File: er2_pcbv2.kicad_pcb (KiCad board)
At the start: 2 copper layers, 83.8 x 57.5 mm, 52 parts, among them IC1 LM2596S, IC2 XC6206, IC3 L293DD, IC4 L293DD, IC5 MMA7455, P1 CONN_3X2, P10 CONN_5, P2 CONN_3X2, P3 CONN_13X2, P4 CONN_2, P5 CONN_2, P6 CONN_2, P7 CONN_2, P8 CONN_2, P9 CONN_2, U1 74HC595

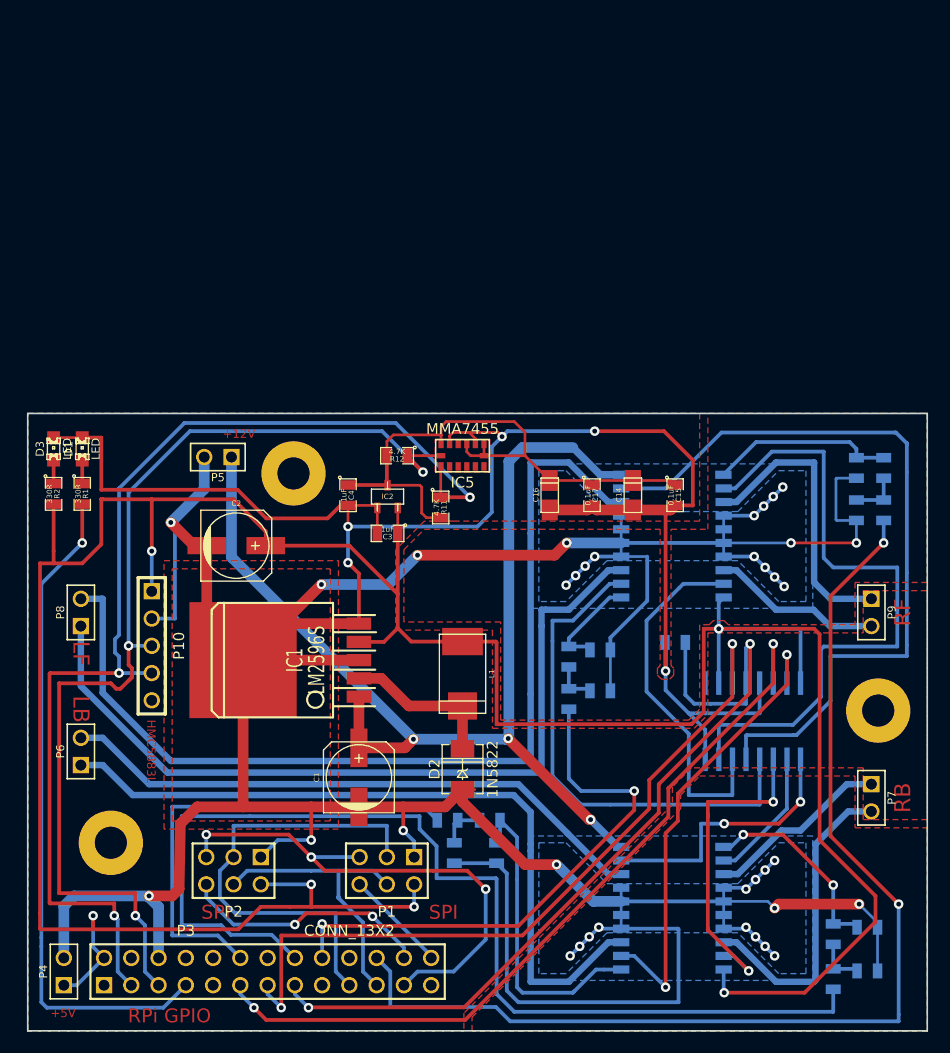
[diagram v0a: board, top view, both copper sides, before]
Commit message: preliminary PCB components placement
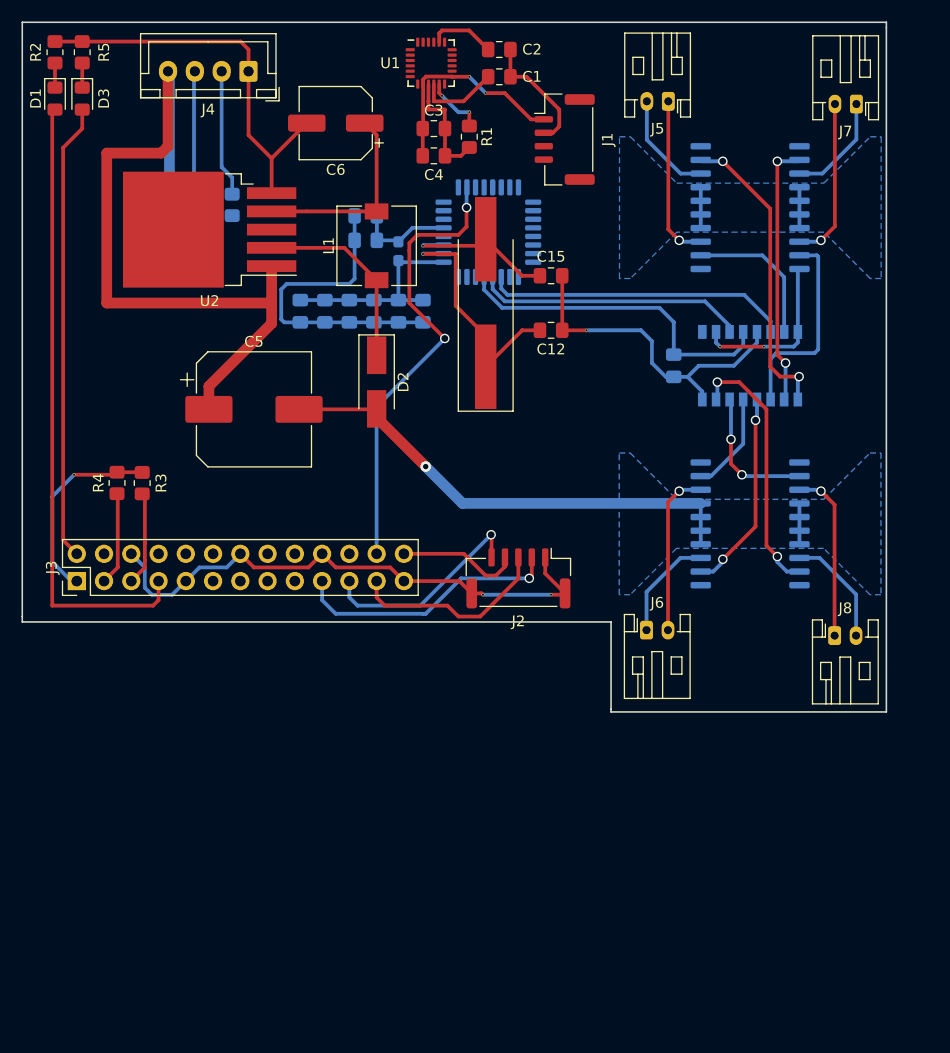
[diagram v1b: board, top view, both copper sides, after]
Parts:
- removed ? (x3): , mnt_hole
- removed IC1: LM2596S, TO263-5
- removed IC2: XC6206, sot23
- removed IC3, IC4: L293DD, -SO20-2
- removed IC5: MMA7455, LGA_14
- removed P1, P2: CONN_3X2, pin_array_3x2
- removed P10: CONN_5, PIN_ARRAY_5x1
- removed P3: CONN_13X2, pin_array_13x2
- removed P4, P5, P6, P7, P8, P9: CONN_2, PIN_ARRAY_2X1
- removed R11, R12: 4.7K, SM0805
- added J1: HMC5883L, Connector_JST:JST_GH_BM04B-GHS-TBT_1x04-1MP_P1.25mm_Vertical, F.Cu at (158.0, 50.8)
- added J2: SPI1, Connector_JST:JST_GH_BM05B-GHS-TBT_1x05-1MP_P1.25mm_Vertical, F.Cu at (153.7, 91.7)
- added J3: raspberry_b_plus_header, Connector_PinHeader_2.54mm:PinHeader_2x13_P2.54mm_Vertical, F.Cu at (112.5, 91.9)
- added J4: Power, Connector_JST:JST_XH_B4B-XH-A_1x04_P2.50mm_Vertical, F.Cu at (128.5, 44.5)
- added J5: WHL_LF, Connector_JST:JST_PH_S2B-PH-K_1x02_P2.00mm_Horizontal, F.Cu at (167.6, 47.2)
- added J6: WHL_LB, Connector_JST:JST_PH_S2B-PH-K_1x02_P2.00mm_Horizontal, F.Cu at (165.6, 96.5)
- added J7: WHL_RF, Connector_JST:JST_PH_S2B-PH-K_1x02_P2.00mm_Horizontal, F.Cu at (185.2, 47.5)
- added J8: WHL_RB, Connector_JST:JST_PH_S2B-PH-K_1x02_P2.00mm_Horizontal, F.Cu at (183.1, 97.0)
- added L2: 39nH, Inductor_SMD:L_0603_1608Metric_Pad1.05x0.95mm_HandSolder, B.Cu at (142.5, 61.2)
- added U2: LM2596S-5, Package_TO_SOT_SMD:TO-263-5_TabPin3, F.Cu at (124.9, 59.2)
- added U3: STM32F030K6Tx, Package_QFP:LQFP-32_7x7mm_P0.8mm, B.Cu at (150.9, 59.4)
- added U4: 74HC595, Package_SO:SOP-16_4.4x10.4mm_P1.27mm, B.Cu at (175.3, 71.9)
- added U5: L293DD, Package_SO:SOP-20_7.5x12.8mm_P1.27mm, B.Cu at (175.3, 57.1)
- added U6: L293DD, Package_SO:SOP-20_7.5x12.8mm_P1.27mm, B.Cu at (175.3, 86.6)
- added Y1: 8Mhz, Crystal:Crystal_SMD_HC49-SD_HandSoldering, F.Cu at (150.6, 66.0)
- C1: value 100uF -> 0.1uF; footprint c_elec_6.3x7.7 -> Capacitor_SMD:C_0805_2012Metric_Pad1.18x1.45mm_HandSolder
- C10, C8, C9: value 1uF -> 100nF; footprint SM0805 -> Capacitor_SMD:C_0805_2012Metric_Pad1.18x1.45mm_HandSolder
- C11: footprint SM0805 -> Capacitor_SMD:C_0805_2012Metric_Pad1.18x1.45mm_HandSolder
- C12: value 1uF -> 20p; footprint SM0805 -> Capacitor_SMD:C_0805_2012Metric_Pad1.18x1.45mm_HandSolder; moved to F.Cu
- C13: value 0.1uF -> 100nF; footprint SM0805 -> Capacitor_SMD:C_0805_2012Metric_Pad1.18x1.45mm_HandSolder
- C14: value 10uF -> 10nF; footprint c_tant_A -> Capacitor_SMD:C_0805_2012Metric_Pad1.18x1.45mm_HandSolder; moved to B.Cu
- C15: value 0.1uF -> 20p; footprint SM0805 -> Capacitor_SMD:C_0805_2012Metric_Pad1.18x1.45mm_HandSolder
- C16: value 10uF -> 100nF; footprint c_tant_A -> Capacitor_SMD:C_0805_2012Metric_Pad1.18x1.45mm_HandSolder; moved to B.Cu
- C17: value 0.1uF -> 1uF; footprint SM0805 -> Capacitor_SMD:C_0805_2012Metric_Pad1.18x1.45mm_HandSolder; moved to B.Cu
- C2: value 220uF -> 2.2nF; footprint c_elec_6.3x7.7 -> Capacitor_SMD:C_0805_2012Metric_Pad1.18x1.45mm_HandSolder
- C3: value 1uF -> 10nF; footprint SM0805 -> Capacitor_SMD:C_0805_2012Metric_Pad1.18x1.45mm_HandSolder
- C4: value 1uF -> 0.1uF; footprint SM0805 -> Capacitor_SMD:C_0805_2012Metric_Pad1.18x1.45mm_HandSolder
- C5: value 1uF -> 680uF; footprint SM0805 -> Capacitor_SMD:CP_Elec_10x10.5; moved to F.Cu
- C6: value 1uF -> 220uF; footprint SM0805 -> Capacitor_SMD:CP_Elec_6.3x7.7; moved to F.Cu
- C7: value 1uF -> 4.7uF; footprint SM0805 -> Capacitor_SMD:C_0805_2012Metric_Pad1.18x1.45mm_HandSolder
- D1, D3: footprint LED-0805 -> LED_SMD:LED_0805_2012Metric_Pad1.15x1.40mm_HandSolder
- D2: footprint DO-214AC(SMA) -> Diode_SMD:D_SMA_Handsoldering
- L1: footprint c_tant_X -> Inductor_SMD:L_7.3x7.3_H3.5
- R1, R2: value 330R -> 1k; footprint SM0805 -> Resistor_SMD:R_0805_2012Metric_Pad1.20x1.40mm_HandSolder
- R10, R7, R8: value 4.7K -> 10k; footprint SM0805 -> Resistor_SMD:R_0805_2012Metric_Pad1.20x1.40mm_HandSolder
- R3, R4: value 4.7K -> 4.7k; footprint SM0805 -> Resistor_SMD:R_0805_2012Metric_Pad1.20x1.40mm_HandSolder; moved to F.Cu
- R5: value 4.7K -> 1k; footprint SM0805 -> Resistor_SMD:R_0805_2012Metric_Pad1.20x1.40mm_HandSolder; moved to F.Cu
- R6, R9: value 4.7K -> 22k; footprint SM0805 -> Resistor_SMD:R_0805_2012Metric_Pad1.20x1.40mm_HandSolder
- U1: value 74HC595 -> MPU-6050; footprint -SOP-16 -> Sensor_Motion:InvenSense_QFN-24_4x4mm_P0.5mm; moved to F.Cu
- moved C6 93.2 mm to (136.7, 49.3), turned to 180 degrees
- moved R8 87.5 mm to (123.4, 60.7), turned to 270 degrees
- moved R4 81.2 mm to (116.3, 82.8), turned to 270 degrees
- moved R5 75.4 mm to (113.0, 42.7)
- moved C10 75.0 mm to (137.9, 66.8), turned to 270 degrees
- moved R10 69.7 mm to (121.2, 60.7), turned to 270 degrees
- moved U1 68.2 mm to (145.5, 43.7), turned to 0 degrees
- moved R6 67.0 mm to (127.0, 56.9), turned to 270 degrees
- moved C1 66.6 mm to (151.9, 45.0), turned to 0 degrees
- moved R7 63.6 mm to (123.4, 56.9), turned to 270 degrees
- moved R9 56.2 mm to (121.2, 56.9), turned to 270 degrees
- moved C2 52.3 mm to (151.9, 42.4)
- moved C9 51.8 mm to (140.2, 66.8)
- moved R1 49.1 mm to (149.1, 50.5)
- moved C8 46.5 mm to (142.5, 66.8)
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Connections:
- C1 pad 1: +12V -> Net-(C1-Pad1)
- C10 pad 1: /DC-motors drivers/pwm2_f -> MPU6050_VDD
- C11 pad 1: /DC-motors drivers/pwm3_f -> +3.3VA
- C12 pad 1: /DC-motors drivers/pwm4_f -> HSE_IN
- C13 pad 1: /DC-motors drivers/RCLK -> MPU6050_VDD
- C14 pad 1: +3.3V -> +3.3VA
- C15 pad 1: +3.3V -> HSE_OUT
- C16 pad 1: +3.3V -> MPU6050_VDD
- C17 pad 1: +3.3V -> WHL_RCLK
- C2 pad 1: +5V -> Net-(C2-Pad1)
- C3 pad 1: +5V -> MPU6050_VDD
- C4 pad 1: +3.3V -> MPU6050_VDD
- C5 pad 1: N-0000056 -> +12V
- C6 pad 1: N-0000054 -> +5V
- C7 pad 1: N-0000055 -> MPU6050_VDD
- C8 pad 1: N-0000036 -> MPU6050_VDD
- C9 pad 1: /DC-motors drivers/pwm1_f -> MPU6050_VDD
- D1 pad 1: N-0000028 -> Net-(D1-Pad1)
- D1 pad 2: GND -> SIGNAL_LED
- D2 pad 1: GND -> Net-(D2-Pad1)
- D2 pad 2: N-0000032 -> GND
- D3 pad 1: N-0000030 -> Net-(D3-Pad1)
- D3 pad 2: GND -> +5V
- L1 pad 1: N-0000032 -> Net-(D2-Pad1)
- R1 pad 1: N-0000028 -> Net-(R1-Pad1)
- R1 pad 2: N-0000022 -> GND
- R10 pad 1: N-0000036 -> BAT3
- R10 pad 2: /DC-motors drivers/pwm4_f -> GND
- R2 pad 1: N-0000030 -> Net-(D1-Pad1)
- R2 pad 2: +5V -> GND
- R3 pad 1: /DC-motors drivers/pwm1 -> MPU6050_VDD
- R3 pad 2: N-0000056 -> SCL
- R4 pad 1: /DC-motors drivers/pwm2 -> MPU6050_VDD
- R4 pad 2: N-0000054 -> SDA
- R5 pad 1: /DC-motors drivers/pwm3 -> Net-(D3-Pad1)
- R5 pad 2: N-0000055 -> GND
- R6 pad 1: /DC-motors drivers/pwm4 -> Net-(J4-Pad2)
- R6 pad 2: N-0000036 -> BAT1
- R7 pad 1: N-0000056 -> Net-(J4-Pad3)
- R7 pad 2: /DC-motors drivers/pwm1_f -> BAT2
- R8 pad 1: N-0000054 -> BAT2
- R8 pad 2: /DC-motors drivers/pwm2_f -> GND
- R9 pad 1: N-0000055 -> +12V
- R9 pad 2: /DC-motors drivers/pwm3_f -> BAT3
- U1 pad 1: N-0000034 -> GND
- U1 pad 10: +5V -> Net-(C1-Pad1)
- U1 pad 11: /DC-motors drivers/SRCLK -> Net-(R1-Pad1)
- U1 pad 12: /DC-motors drivers/RCLK -> (no net)
- U1 pad 13: GND -> MPU6050_VDD
- U1 pad 14: /DC-motors drivers/SER -> (no net)
- U1 pad 15: N-0000035 -> (no net)
- U1 pad 16: +5V -> (no net)
- U1 pad 2: N-0000047 -> (no net)
- U1 pad 3: N-0000033 -> (no net)
- U1 pad 4: N-0000040 -> (no net)
- U1 pad 5: N-0000043 -> (no net)
- U1 pad 6: N-0000041 -> AUXSDA
- U1 pad 7: N-0000046 -> AUXSCL
- U1 pad 8: GND -> MPU6050_VDD
- U1 pad 9: (no net) -> GND
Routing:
- net GND: track 533.4 -> 231.2 mm, vias 41 -> 4
- net +5V: track 288.1 -> 61.1 mm, vias 6 -> 0
- net /Accelerometer/SDA: track 106.5 -> 0.00 mm, vias 3 -> 0
- net /DC-motors drivers/pwm4: track 104.3 -> 0.00 mm, vias 2 -> 0
- net /DC-motors drivers/pwm2: track 101.1 -> 0.00 mm
- net /Accelerometer/SCL: track 100.2 -> 0.00 mm, vias 3 -> 0
- net N-0000044: track 91.1 -> 0.00 mm
- net /DC-motors drivers/RCLK: track 78.7 -> 0.00 mm, vias 2 -> 0
- net N-0000045: track 76.0 -> 0.00 mm
- net MPU6050_VDD: track 0.00 -> 73.8 mm, vias 0 -> 5
- net /DC-motors drivers/SER: track 73.4 -> 0.00 mm, vias 2 -> 0
- net N-0000043: track 71.9 -> 0.00 mm
- net /DC-motors drivers/SRCLK: track 70.8 -> 0.00 mm, vias 2 -> 0
- net N-0000049: track 69.5 -> 0.00 mm
- net N-0000022: track 62.5 -> 0.00 mm, vias 1 -> 0
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- removed copper zone on B.Cu, net (none)
- removed copper zone on F.Cu, net (none)
- removed copper zone on F.Cu, net GND
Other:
- board size 83.8 x 57.5 mm -> 80.5 x 64.3 mm
- net class acc_sig added: clearance 0.01, trace_width 0.35, via_dia 0.254, via_drill 0.2
- rule via_min_drill: 0.508 -> 0.2
- rule via_min_size: 0.889 -> 0.254
- board text removed: "+12V"
- board text removed: "+5V"
- board text removed: "HMC5883L"
- board text removed: "LB"
- board text removed: "LF"
- board text removed: "RB"
- board text removed: "RF"
- board text removed: "RPi GPIO"
- board text removed: "SPI"
